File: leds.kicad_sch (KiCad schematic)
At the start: 107 parts, among them IC1 HT16K33, J36 Conn_01x04, J40 Conn_01x04, U3 SA39-12SRWA, U4 SA39-12SRWA, U5 PCA9306DC, U6 PCA9306DP, U7 SA39-12SRWA

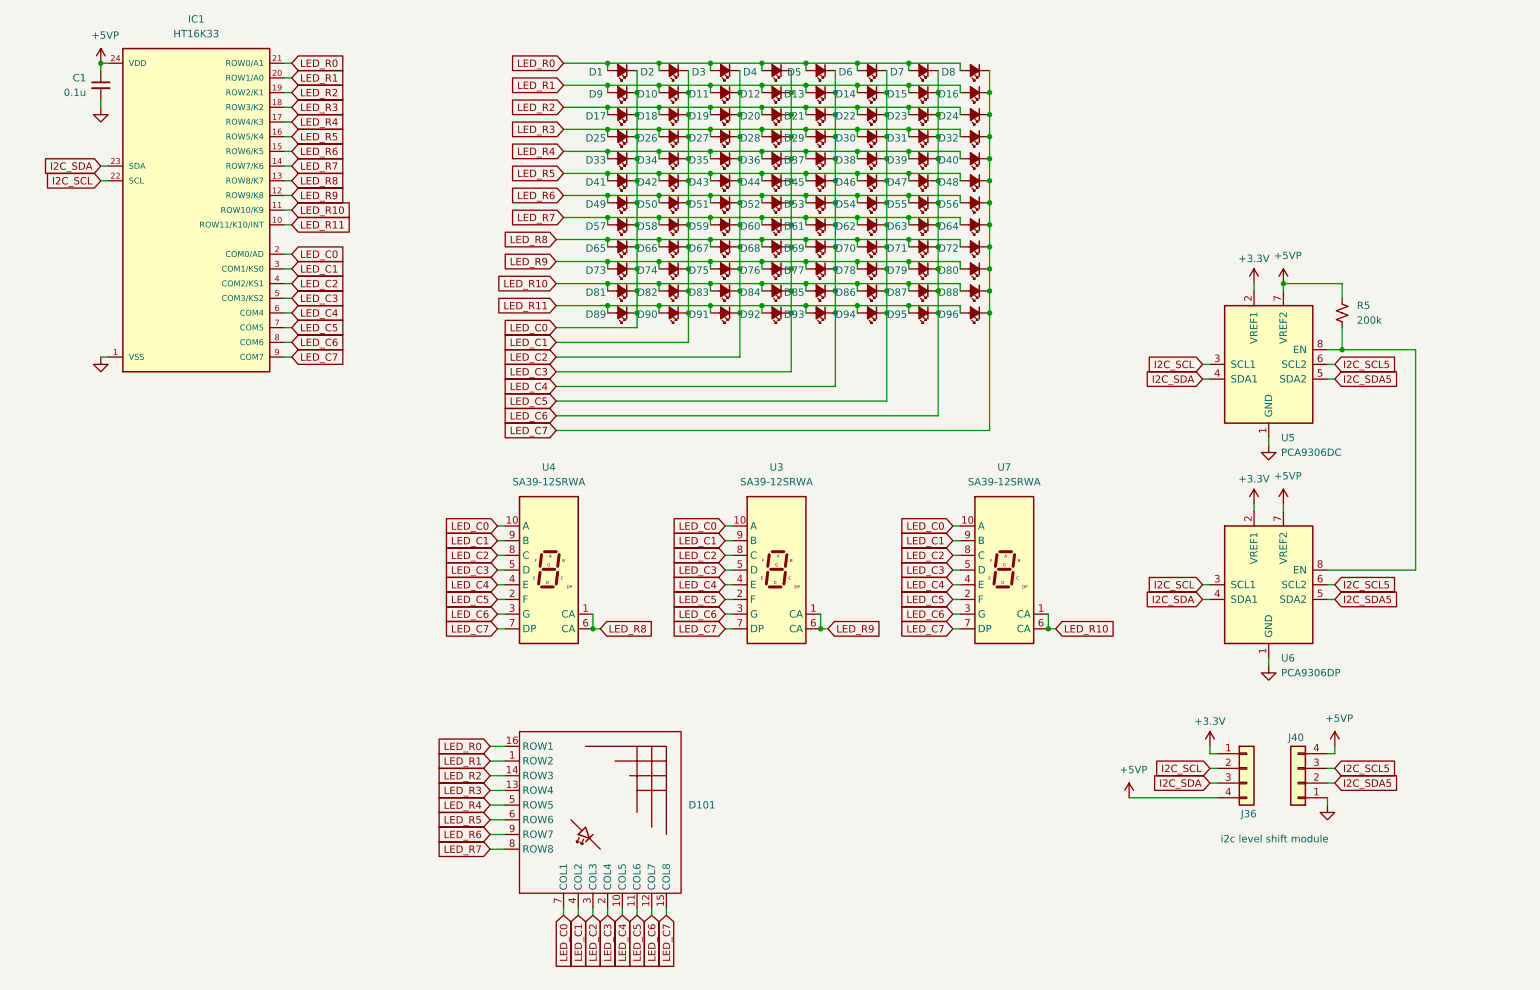
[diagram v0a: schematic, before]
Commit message: 更新
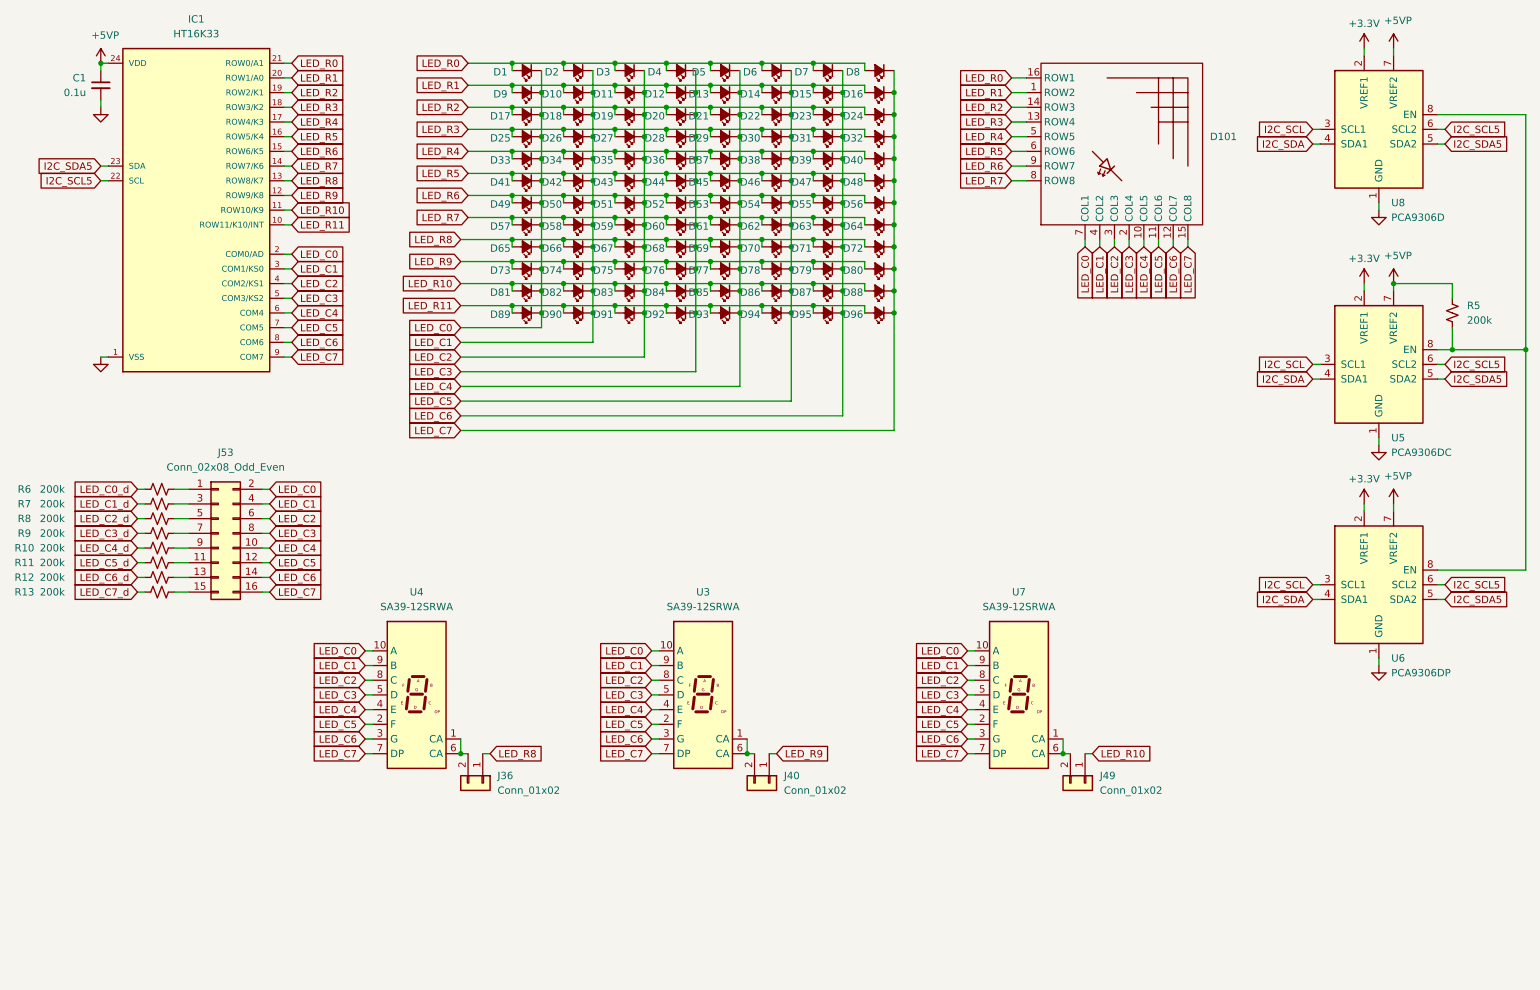
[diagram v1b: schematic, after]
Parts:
- removed J36, J40: Conn_01x04, Connector_PinSocket_2.54mm:PinSocket_1x04_P2.54mm_Vertical, symbol Connector_Generic:Conn_01x04
- added J36, J40, J49: Conn_01x02, Connector_PinHeader_2.54mm:PinHeader_2x01_P2.54mm_Vertical, symbol Connector_Generic:Conn_01x02
- added J53: Conn_02x08_Odd_Even, Connector_PinHeader_2.54mm:PinHeader_2x08_P2.54mm_Vertical, symbol Connector_Generic:Conn_02x08_Odd_Even
- added R10, R11, R12, R13, R6, R7, R8, R9: 200k, Resistor_SMD:R_0402_1005Metric_Pad0.72x0.64mm_HandSolder, symbol Device:R_Small_US
- added U8: PCA9306D, Package_SO:SO-8_3.9x4.9mm_P1.27mm, symbol Interface:PCA9306D
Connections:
- net +3.3V: now also U8.2 (VREF1)
- net +5VP: now also U8.7 (VREF2)
- net GND: now also U8.1 (GND)
- net I2C_SCL: now also U8.3 (SCL1); no longer IC1.22 (SCL)
- net I2C_SCL5: now also IC1.22 (SCL), U8.6 (SCL2)
- net I2C_SDA: now also U8.4 (SDA1); no longer IC1.23 (SDA)
- net I2C_SDA5: now also IC1.23 (SDA), U8.5 (SDA2)
- net LED_C0: now also J53.2 (Pin_2)
- net LED_C1: now also J53.4 (Pin_4)
- net LED_C2: now also J53.6 (Pin_6)
- net LED_C3: now also J53.8 (Pin_8)
- net LED_C4: now also J53.10 (Pin_10)
- net LED_C5: now also J53.12 (Pin_12)
- net LED_C6: now also J53.14 (Pin_14)
- net LED_C7: now also J53.16 (Pin_16)
- net LED_R10: now also J49.1 (Pin_1); no longer U7.1 (CA), U7.6 (CA)
- net LED_R8: now also J36.1 (Pin_1); no longer U4.1 (CA), U4.6 (CA)
- net LED_R9: now also J40.1 (Pin_1); no longer U3.1 (CA), U3.6 (CA)
- net at R5.1, U5.8 (EN), U6.8 (EN): now also U8.8 (EN)
- new net: J49.2 (Pin_2), U7.1 (CA), U7.6 (CA)
- new net: J53.5 (Pin_5), R8.1
- new net: J53.15 (Pin_15), R13.1
- new net: J40.2 (Pin_2), U3.1 (CA), U3.6 (CA)
- new net: J53.9 (Pin_9), R10.1
- new net: J53.13 (Pin_13), R12.1
- new net: J36.2 (Pin_2), U4.1 (CA), U4.6 (CA)
- new net: J53.3 (Pin_3), R7.1
- new net: J53.1 (Pin_1), R6.1
- new net: J53.11 (Pin_11), R11.1
- new net: J53.7 (Pin_7), R9.1
- new net LED_C0_d: R6.2
- new net LED_C1_d: R7.2
- new net LED_C2_d: R8.2
- new net LED_C3_d: R9.2
- new net LED_C4_d: R10.2
- new net LED_C5_d: R11.2
- new net LED_C6_d: R12.2
- new net LED_C7_d: R13.2
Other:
- note removed: "i2c level shift module"
- moved on the sheet: D1, D10, D101, D11, D12, D13, D14, D15, D16, D17, D18, D19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
